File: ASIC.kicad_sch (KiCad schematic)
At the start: 86 parts, among them U10 TLV77308PDBVR, U11 TLV77312PDBVR, U12 TLV77308PDBVR, U14 TLV77312PDBVR, U15 25MHz, U2 SN74AVC4T774, U8 25MHz

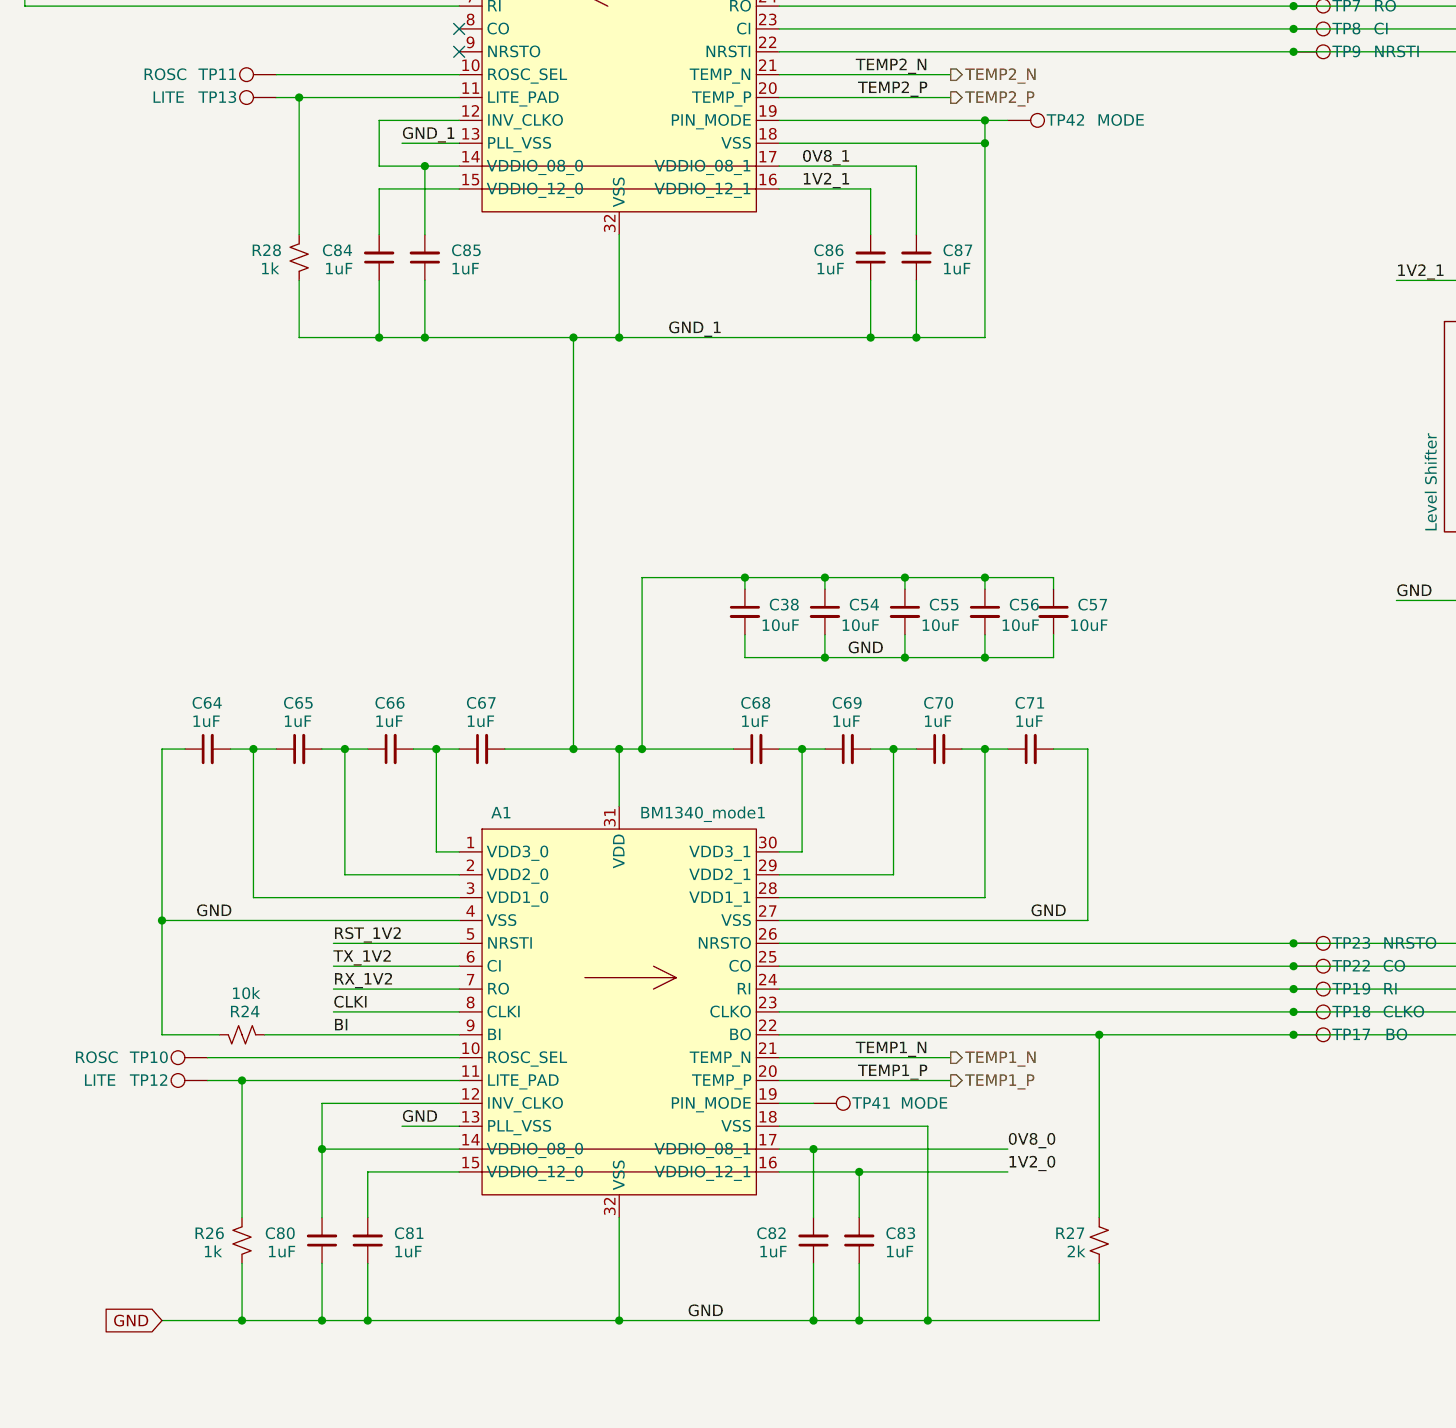
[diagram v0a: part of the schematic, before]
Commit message: finished routing
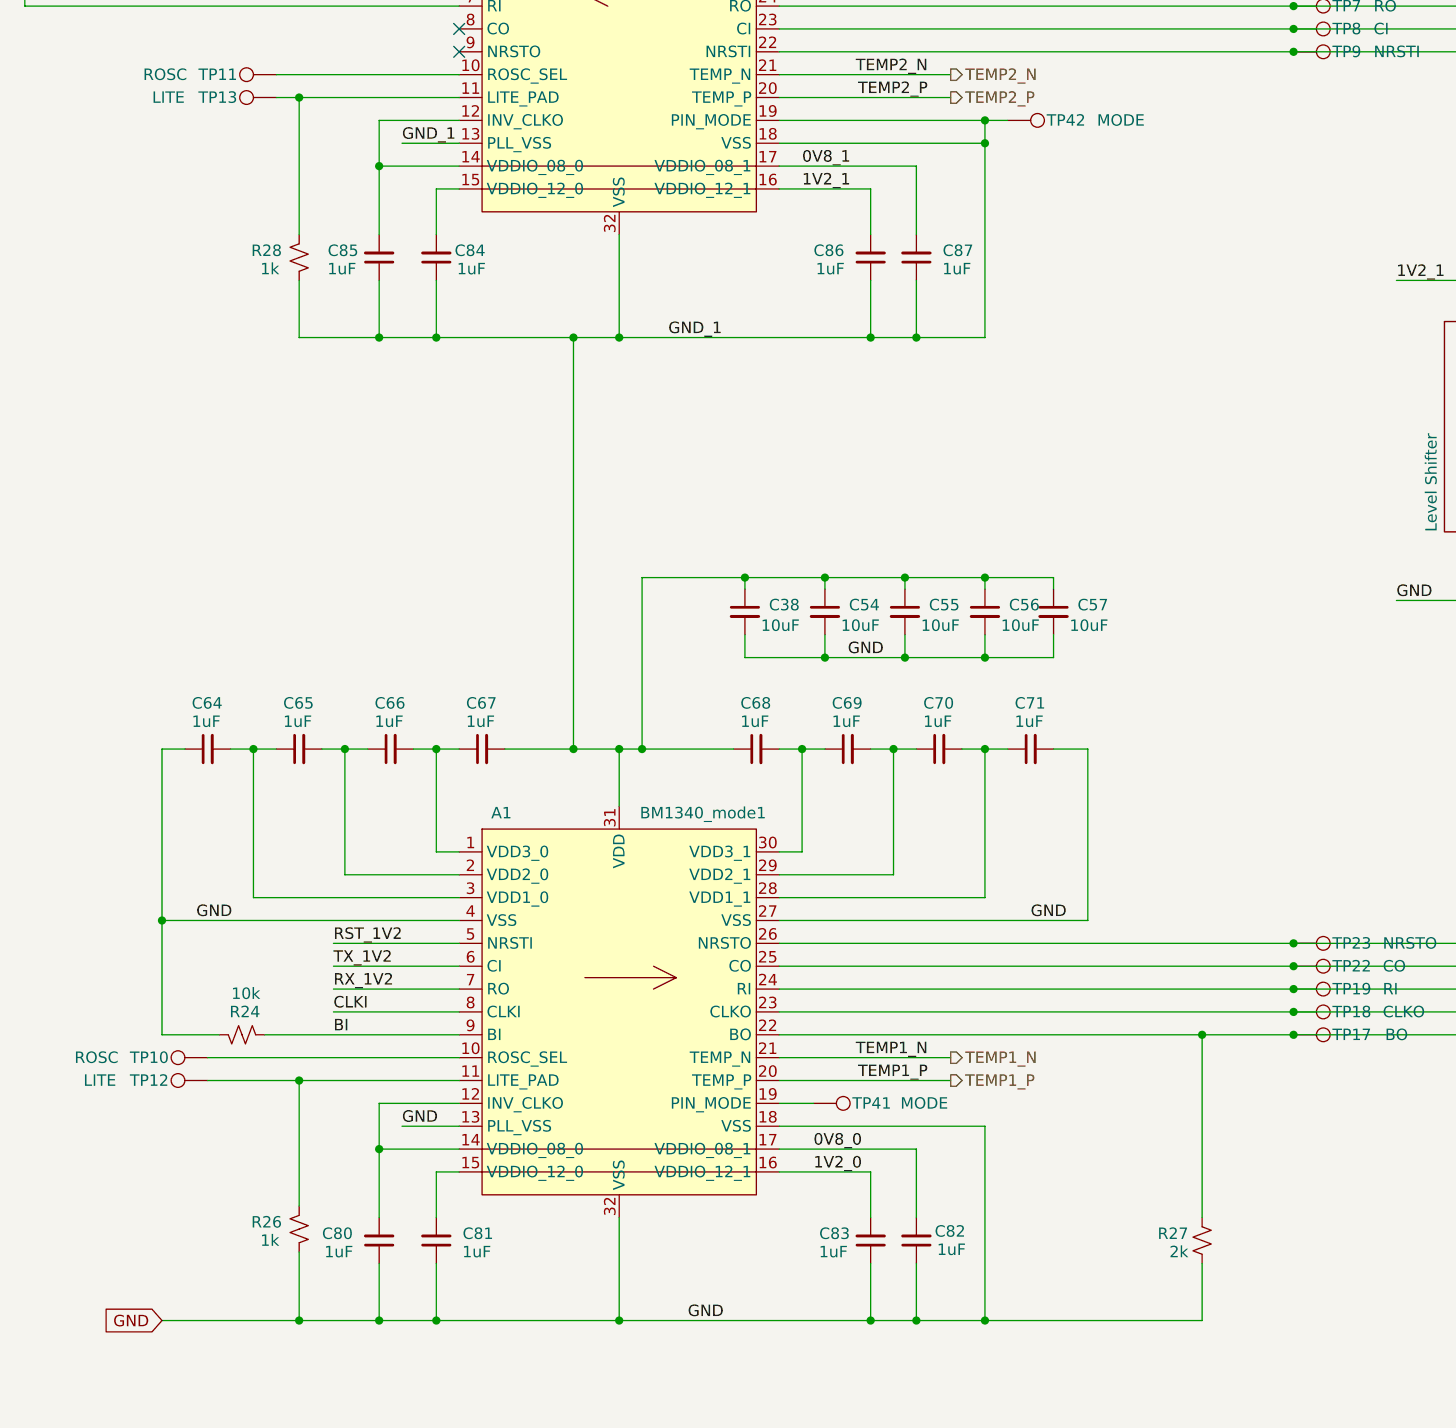
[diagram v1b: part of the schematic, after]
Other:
- moved on the sheet: C80, C81, C82, C83, C84, C85, R26, R27
